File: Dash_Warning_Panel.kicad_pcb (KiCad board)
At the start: 2 copper layers, 57.5 x 40 mm, 42 parts, among them J1 Conn, U1 TLC6C5816, U2 TPS22810

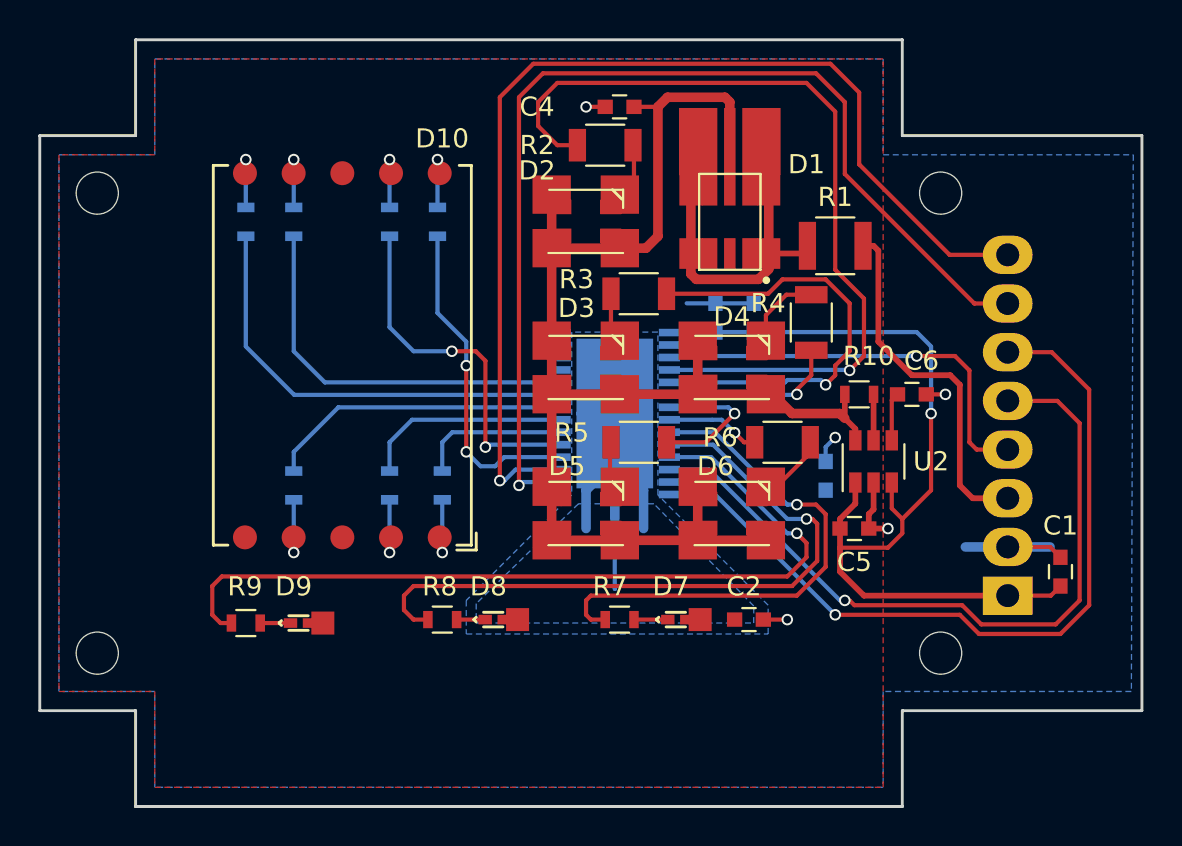
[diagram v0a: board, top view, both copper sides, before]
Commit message: First Manufacture Ready 2020
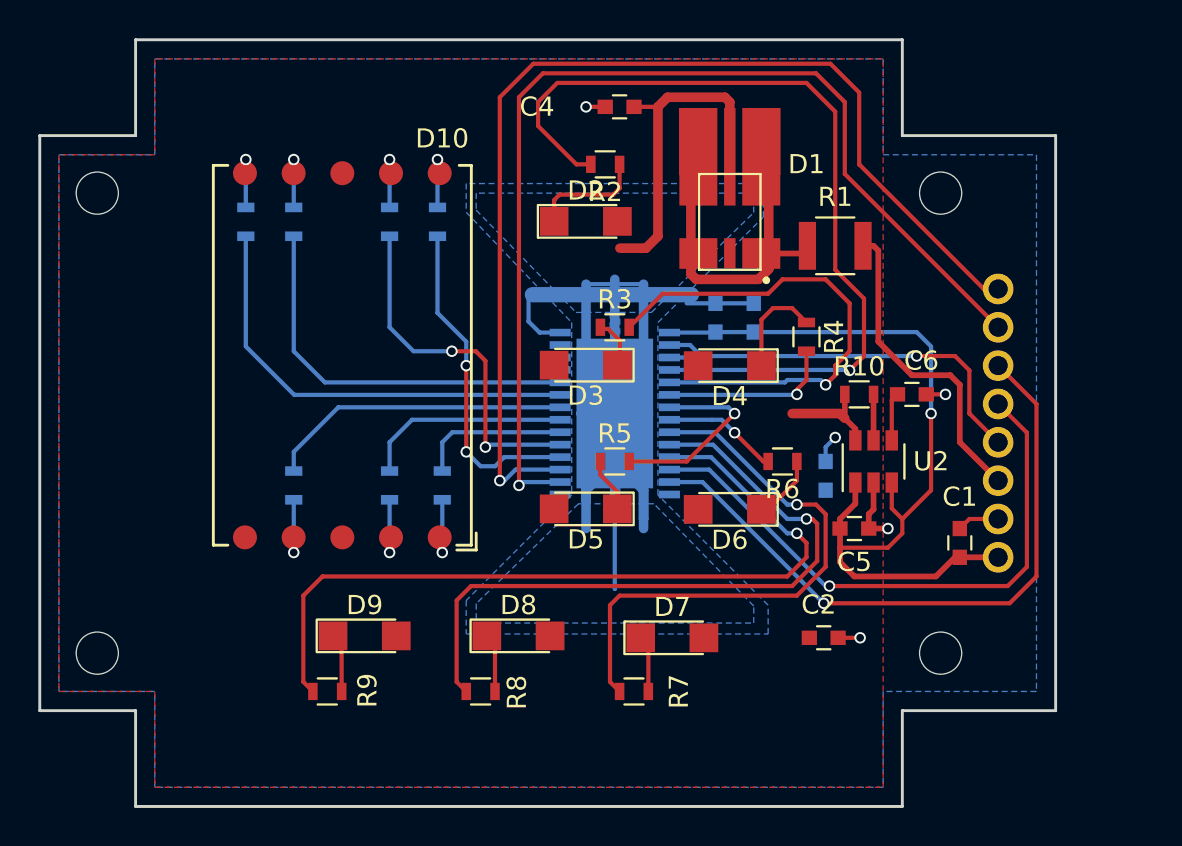
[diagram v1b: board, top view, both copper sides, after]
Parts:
- D2, D6: value LY E6SF -> SM1206NYC-IL; footprint OSRAM:OSRAM_PLCC-4_THERM_PAD -> LEDs:LED_1206
- D3, D4, D5: value LS E6SF -> SM1206NHC-IL; footprint OSRAM:OSRAM_PLCC-4_THERM_PAD -> LEDs:LED_1206
- D7, D8, D9: value KP DELPS -> SM1206NPGC-IL; footprint OSRAM:PLCC-2 -> LEDs:LED_1206
- J1: footprint Molex:Molex_KK-171857_08x2.54mm_Right_Angle -> FSAE-Dash-Warning-Panel:8wireConn
- R1: value 11.3 -> 11
- R10: value 86.6 -> 120
- R11, R12, R13, R14, R15, R16, R17, R7, R8, R9: value 116.7 -> 120
- R2, R3, R4, R5, R6: value 71 -> 120; footprint Resistors_SMD:R_1206 -> Resistors_SMD:R_0603
- moved R9 5.55 mm to (184.0, 142.0)
- moved C1 5.46 mm to (217.0, 134.2)
- moved R8 4.25 mm to (192.0, 142.0)
- moved C2 4.01 mm to (209.9, 139.2)
- moved R7 3.82 mm to (200.0, 142.0)
- moved D9 3.77 mm to (185.9, 139.1)
- moved R3 2.15 mm to (199.0, 123.0)
- moved J1 2.06 mm to (219.0, 135.0), turned to 0 degrees
- moved D8 1.79 mm to (194.0, 139.1)
- moved R5 1.60 mm to (199.0, 130.0)
- moved R2 1.00 mm to (198.5, 114.5)
- moved R6 1.00 mm to (207.8, 130.0)
- moved D7 0.95 mm to (202.0, 139.2)
- moved R4 0.79 mm to (209.0, 123.5)
- moved D5 0.24 mm to (197.5, 132.5), turned to 180 degrees
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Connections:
- U1 pad 29: Net-(U1-Pad26) -> GND
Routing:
- net GND: track 18.0 -> 76.5 mm
- net /LED_Power: track 77.2 -> 25.8 mm
- net Net-(U1-Pad26): track 16.7 -> 0.00 mm
- net /SDI: track 38.7 -> 30.7 mm
- net /CLR: track 42.1 -> 34.2 mm
- net /VCC: track 47.2 -> 43.5 mm
- net /D2_h: track 2.90 -> 6.03 mm
- net /D3: track 23.5 -> 26.1 mm
- net /D5: track 7.71 -> 10.1 mm
- net /NEUT: track 18.9 -> 16.7 mm
- net /D9: track 44.1 -> 42.0 mm
- net /D9_h: track 1.58 -> 3.30 mm
- net /D7: track 27.7 -> 29.5 mm
- net /D8_h: track 1.49 -> 3.08 mm
- net /G: track 23.8 -> 22.3 mm
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- removed copper zone on B.Cu, net Net-(U1-Pad26)
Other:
- board size 57.5 x 40 mm -> 53 x 40 mm
- board text added: "CLR"
- board text added: "CONT"
- board text added: "GND"
- board text added: "NEUT"
- board text added: "RCLK"
- board text added: "SCLK"
- board text added: "SDI"
- board text added: "VCC"
- board text removed: "M2 2.2mm"
- board text removed: "SCLK RCLK CLR SDI CONT NEUT GND VCC"
- board text removed: "Y"
